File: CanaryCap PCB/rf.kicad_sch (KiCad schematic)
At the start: 3 parts

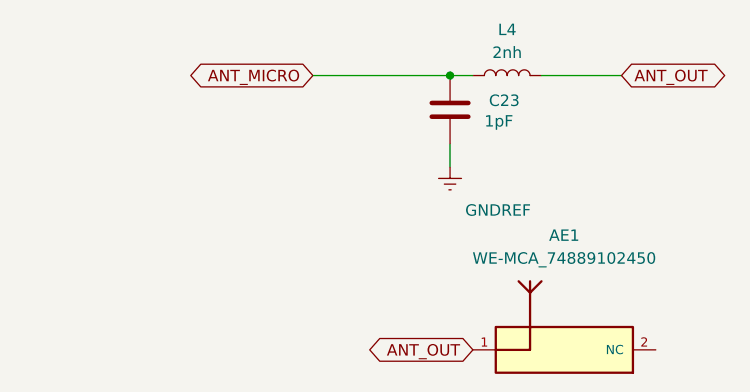
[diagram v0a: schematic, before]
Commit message: YIPPEE
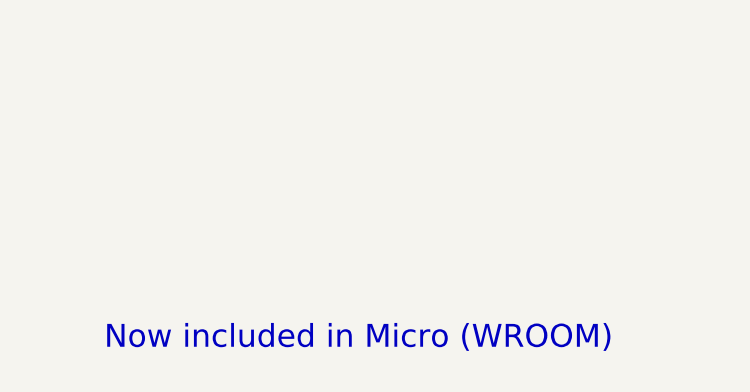
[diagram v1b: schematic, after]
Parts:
- removed AE1: WE-MCA_74889102450, Library:WE-MCA_74889102450, symbol ESP-32-C6:WE-MCA_74889102450
- removed C23: 1pF, Capacitor_SMD:C_0603_1608Metric_Pad1.08x0.95mm_HandSolder, symbol Device:C
- removed L4: 2nh, Inductor_SMD:L_0603_1608Metric, symbol Device:L
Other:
- note added: "Now included in Micro (WROOM)"
